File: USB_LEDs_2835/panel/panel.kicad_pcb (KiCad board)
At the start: 2 copper layers, 99.9 x 120 mm, 280 parts, among them U1 MT9284_1, U2 JL8022W-L, U3 74LVC1G04

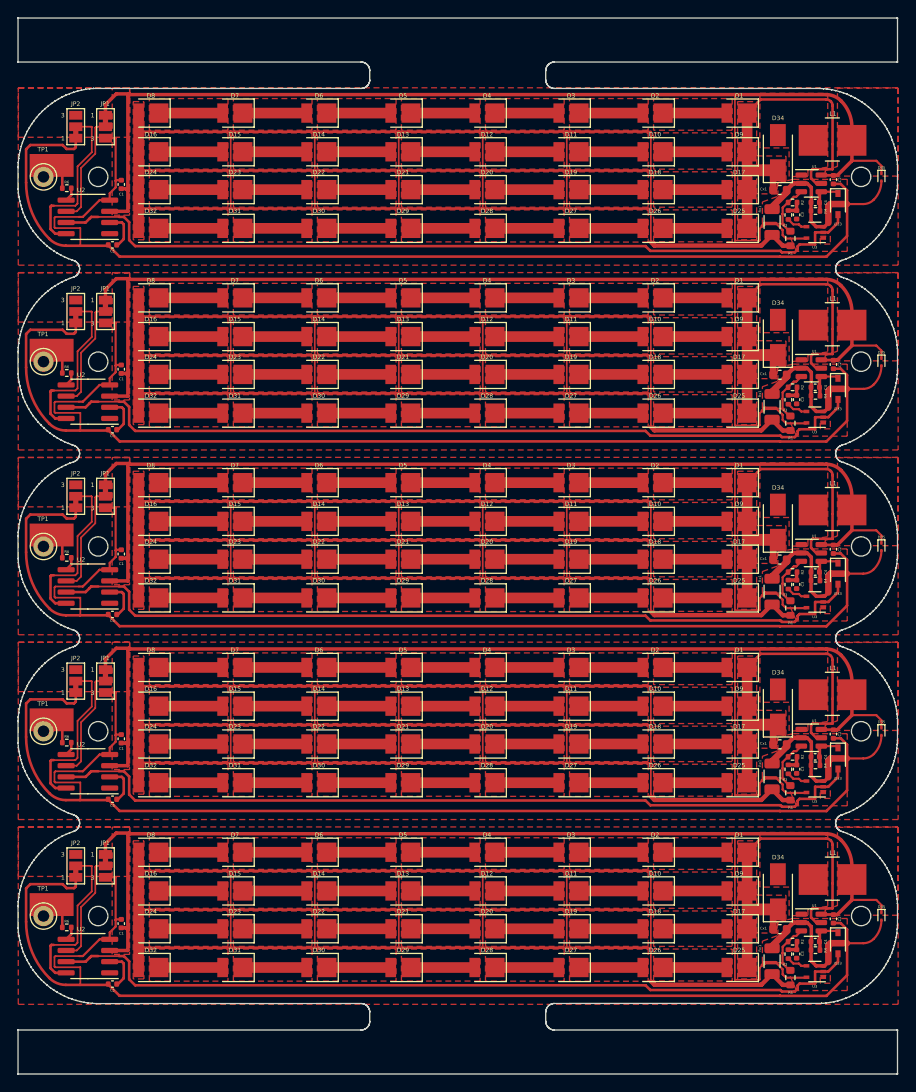
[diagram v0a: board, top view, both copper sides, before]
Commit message: Add files via upload
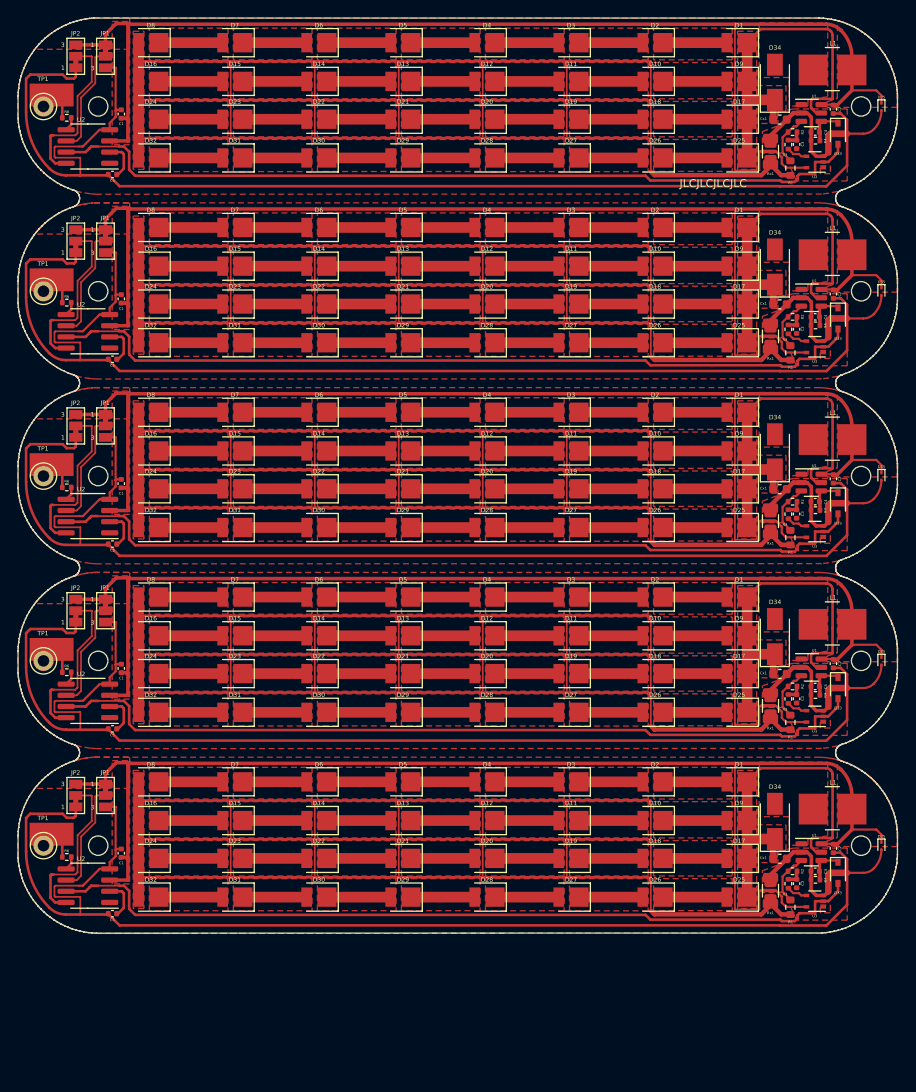
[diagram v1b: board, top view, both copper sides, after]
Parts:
- removed the C1 at (110.3, 59.9)
- removed the C1 at (110.3, 80.9)
- removed the C1 at (110.3, 38.9)
- removed the C1 at (110.3, 122.9)
- removed the C1 at (110.3, 101.9)
- removed the C2 at (191.2, 122.4)
- removed the C2 at (191.2, 38.4)
- removed the C2 at (191.2, 59.4)
- removed the C2 at (191.2, 101.4)
- removed the C2 at (191.2, 80.4)
- removed the C3 at (187.0, 63.4)
- removed the C3 at (187.0, 42.4)
- removed the C3 at (187.0, 105.4)
- removed the C3 at (187.0, 84.4)
- removed the C3 at (187.0, 126.4)
- removed the C4 at (189.1, 41.0)
- removed the C4 at (189.1, 62.0)
- removed the C4 at (189.1, 83.0)
- removed the C4 at (189.1, 104.0)
- removed the C4 at (189.1, 125.0)
- removed the C5 at (109.3, 129.8)
- removed the C5 at (109.3, 87.8)
- removed the C5 at (109.3, 108.8)
- removed the C5 at (109.3, 45.8)
- removed the C5 at (109.3, 66.8)
- removed the Cx1 at (185.1, 81.5)
- removed the Cx1 at (185.1, 123.5)
- removed the Cx1 at (185.1, 60.5)
- removed the Cx1 at (185.1, 39.5)
- removed the Cx1 at (185.1, 102.5)
- removed the D1 at (180.5, 114.8)
- removed the D1 at (180.5, 30.8)
- removed the D1 at (180.5, 72.8)
- removed the D1 at (180.5, 51.8)
- removed the D1 at (180.5, 93.8)
- removed the D10 at (170.9, 35.2)
- removed the D10 at (170.9, 77.2)
- removed the D10 at (170.9, 98.2)
- removed the D10 at (170.9, 119.2)
- removed the D10 at (170.9, 56.2)
- removed the D11 at (161.4, 35.2)
- removed the D11 at (161.4, 119.2)
- removed the D11 at (161.4, 56.2)
- removed the D11 at (161.4, 98.2)
- removed the D11 at (161.4, 77.2)
- removed the D12 at (151.8, 119.2)
- removed the D12 at (151.8, 77.2)
- removed the D12 at (151.8, 56.2)
- removed the D12 at (151.8, 98.2)
- removed the D12 at (151.8, 35.2)
- removed the D13 at (142.3, 77.2)
- removed the D13 at (142.3, 56.2)
- removed the D13 at (142.3, 98.2)
- removed the D13 at (142.3, 35.2)
- removed the D13 at (142.3, 119.2)
- removed the D14 at (132.7, 35.2)
- removed the D14 at (132.7, 98.2)
- removed the D14 at (132.7, 56.2)
- removed the D14 at (132.7, 119.2)
- removed the D14 at (132.7, 77.2)
- removed the D15 at (123.2, 119.2)
- removed the D15 at (123.2, 98.2)
- removed the D15 at (123.2, 35.2)
- removed the D15 at (123.2, 77.2)
- removed the D15 at (123.2, 56.2)
- removed the D16 at (113.6, 98.2)
- removed the D16 at (113.6, 35.2)
- removed the D16 at (113.6, 77.2)
- removed the D16 at (113.6, 56.2)
- removed the D16 at (113.6, 119.2)
- removed the D17 at (180.5, 39.5)
- removed the D17 at (180.5, 102.5)
- removed the D17 at (180.5, 123.5)
- removed the D17 at (180.5, 81.5)
- removed the D17 at (180.5, 60.5)
- removed the D18 at (170.9, 81.5)
- removed the D18 at (170.9, 123.5)
- removed the D18 at (170.9, 60.5)
- removed the D18 at (170.9, 102.5)
- removed the D18 at (170.9, 39.5)
- removed the D19 at (161.4, 123.5)
- removed the D19 at (161.4, 102.5)
- removed the D19 at (161.4, 39.5)
- removed the D19 at (161.4, 81.5)
- removed the D19 at (161.4, 60.5)
- removed the D2 at (170.9, 114.8)
- removed the D2 at (170.9, 93.8)
- removed the D2 at (170.9, 72.8)
- removed the D2 at (170.9, 51.8)
- removed the D2 at (170.9, 30.8)
- removed the D20 at (151.8, 81.5)
- removed the D20 at (151.8, 60.5)
- removed the D20 at (151.8, 102.5)
- removed the D20 at (151.8, 39.5)
- removed the D20 at (151.8, 123.5)
- removed the D21 at (142.3, 123.5)
- removed the D21 at (142.3, 39.5)
- removed the D21 at (142.3, 81.5)
- removed the D21 at (142.3, 60.5)
- removed the D21 at (142.3, 102.5)
- removed the D22 at (132.7, 39.5)
- removed the D22 at (132.7, 60.5)
- removed the D22 at (132.7, 81.5)
- removed the D22 at (132.7, 123.5)
- removed the D22 at (132.7, 102.5)
- removed the D23 at (123.2, 39.5)
- removed the D23 at (123.2, 102.5)
- removed the D23 at (123.2, 123.5)
- removed the D23 at (123.2, 81.5)
- removed the D23 at (123.2, 60.5)
- removed the D24 at (113.6, 123.5)
- removed the D24 at (113.6, 102.5)
- removed the D24 at (113.6, 60.5)
- removed the D24 at (113.6, 81.5)
- removed the D24 at (113.6, 39.5)
- removed the D25 at (180.5, 85.9)
- removed the D25 at (180.5, 43.9)
- removed the D25 at (180.5, 106.9)
- removed the D25 at (180.5, 64.9)
- removed the D25 at (180.5, 127.9)
- removed the D26 at (170.9, 106.9)
- removed the D26 at (170.9, 127.9)
- removed the D26 at (170.9, 43.9)
- removed the D26 at (170.9, 64.9)
- removed the D26 at (170.9, 85.9)
- removed the D27 at (161.4, 64.9)
- removed the D27 at (161.4, 43.9)
- removed the D27 at (161.4, 106.9)
- removed the D27 at (161.4, 127.9)
- removed the D27 at (161.4, 85.9)
- removed the D28 at (151.8, 85.9)
- removed the D28 at (151.8, 43.9)
- removed the D28 at (151.8, 106.9)
- removed the D28 at (151.8, 64.9)
- removed the D28 at (151.8, 127.9)
- removed the D29 at (142.3, 85.9)
- removed the D29 at (142.3, 64.9)
- removed the D29 at (142.3, 43.9)
- removed the D29 at (142.3, 127.9)
- removed the D29 at (142.3, 106.9)
- removed the D3 at (161.4, 51.8)
- removed the D3 at (161.4, 30.8)
- removed the D3 at (161.4, 72.8)
- removed the D3 at (161.4, 93.8)
- removed the D3 at (161.4, 114.8)
- removed the D30 at (132.7, 85.9)
- removed the D30 at (132.7, 43.9)
- removed the D30 at (132.7, 64.9)
- removed the D30 at (132.7, 106.9)
- removed the D30 at (132.7, 127.9)
- removed the D31 at (123.2, 85.9)
- removed the D31 at (123.2, 43.9)
- removed the D31 at (123.2, 106.9)
- removed the D31 at (123.2, 64.9)
- removed the D31 at (123.2, 127.9)
- removed the D32 at (113.6, 106.9)
- removed the D32 at (113.6, 127.9)
- removed the D32 at (113.6, 64.9)
- removed the D32 at (113.6, 43.9)
- removed the D32 at (113.6, 85.9)
- removed the D33 at (191.7, 83.0)
- removed the D33 at (191.7, 125.0)
- removed the D33 at (191.7, 104.0)
- removed the D33 at (191.7, 62.0)
- removed the D33 at (191.7, 41.0)
- removed the D34 at (184.9, 98.3)
- removed the D34 at (184.9, 77.3)
- removed the D34 at (184.9, 35.3)
- removed the D34 at (184.9, 56.3)
- removed the D34 at (184.9, 119.3)
- removed the D35 at (196.6, 101.1)
- removed the D35 at (196.6, 38.1)
- removed the D35 at (196.6, 122.1)
- removed the D35 at (196.6, 59.1)
- removed the D35 at (196.6, 80.1)
- removed the D4 at (151.8, 30.8)
- removed the D4 at (151.8, 72.8)
- removed the D4 at (151.8, 51.8)
- removed the D4 at (151.8, 114.8)
- removed the D4 at (151.8, 93.8)
- removed the D5 at (142.3, 93.8)
- removed the D5 at (142.3, 51.8)
- removed the D5 at (142.3, 72.8)
- removed the D5 at (142.3, 114.8)
- removed the D5 at (142.3, 30.8)
- removed the D6 at (132.7, 30.8)
- removed the D6 at (132.7, 72.8)
- removed the D6 at (132.7, 51.8)
- removed the D6 at (132.7, 93.8)
- removed the D6 at (132.7, 114.8)
- removed the D7 at (123.2, 51.8)
- removed the D7 at (123.2, 93.8)
- removed the D7 at (123.2, 114.8)
- removed the D7 at (123.2, 72.8)
- removed the D7 at (123.2, 30.8)
- removed the D8 at (113.6, 72.8)
- removed the D8 at (113.6, 93.8)
- removed the D8 at (113.6, 30.8)
- removed the D8 at (113.6, 51.8)
- removed the D8 at (113.6, 114.8)
- removed the D9 at (180.5, 119.2)
- removed the D9 at (180.5, 98.2)
- removed the D9 at (180.5, 77.2)
- removed the D9 at (180.5, 56.2)
- removed the D9 at (180.5, 35.2)
- removed the H1 at (194.3, 122.0)
- removed the H1 at (194.3, 101.0)
- removed the H1 at (194.3, 80.0)
- removed the H1 at (194.3, 59.0)
- removed the H1 at (194.3, 38.0)
- removed the H2 at (107.7, 59.0)
- removed the H2 at (107.7, 101.0)
- removed the H2 at (107.7, 122.0)
- removed the H2 at (107.7, 38.0)
- removed the H2 at (107.7, 80.0)
- removed the JP1 at (108.5, 95.3)
- removed the JP1 at (108.5, 53.3)
- removed the JP1 at (108.5, 74.3)
- removed the JP1 at (108.5, 32.3)
- removed the JP1 at (108.5, 116.3)
- removed the JP2 at (105.1, 116.3)
- removed the JP2 at (105.1, 95.3)
- removed the JP2 at (105.1, 32.3)
- removed the JP2 at (105.1, 53.3)
- removed the JP2 at (105.1, 74.3)
- removed the L1 at (191.1, 33.9)
- removed the L1 at (191.1, 96.9)
- removed the L1 at (191.1, 54.9)
- removed the L1 at (191.1, 75.9)
- removed the L1 at (191.1, 117.9)
- removed the R1 at (186.3, 108.0)
- removed the R1 at (186.3, 129.0)
- removed the R1 at (186.3, 87.0)
- removed the R1 at (186.3, 66.0)
- removed the R1 at (186.3, 45.0)
- removed the R2 at (186.5, 104.0)
- removed the R2 at (186.5, 62.0)
- removed the R2 at (186.5, 83.0)
- removed the R2 at (186.5, 125.0)
- removed the R2 at (186.5, 41.0)
- removed the R3 at (186.1, 42.4)
- removed the R3 at (186.1, 84.4)
- removed the R3 at (186.1, 126.4)
- removed the R3 at (186.1, 63.4)
- removed the R3 at (186.1, 105.4)
- removed the R4 at (189.1, 41.9)
- removed the R4 at (189.1, 62.9)
- removed the R4 at (189.1, 125.9)
- removed the R4 at (189.1, 104.9)
- removed the R4 at (189.1, 83.9)
- removed the R6 at (104.1, 102.3)
- removed the R6 at (104.1, 39.3)
- removed the R6 at (104.1, 123.3)
- removed the R6 at (104.1, 60.3)
- removed the R6 at (104.1, 81.3)
- removed the Rx1 at (184.2, 106.2)
- removed the Rx1 at (184.2, 43.2)
- removed the Rx1 at (184.2, 85.2)
- removed the Rx1 at (184.2, 127.2)
- removed the Rx1 at (184.2, 64.2)
- removed the TP1 at (101.4, 80.0)
- removed the TP1 at (101.4, 38.0)
- removed the TP1 at (101.4, 59.0)
- removed the TP1 at (101.4, 122.0)
- removed the TP1 at (101.4, 101.0)
- removed the U1 at (188.7, 80.8)
- removed the U1 at (188.7, 38.8)
- removed the U1 at (188.7, 122.8)
- removed the U1 at (188.7, 59.8)
- removed the U1 at (188.7, 101.8)
- removed the U2 at (106.5, 126.6)
- removed the U2 at (106.5, 84.6)
- removed the U2 at (106.5, 63.6)
- removed the U2 at (106.5, 105.6)
- removed the U2 at (106.5, 42.6)
- removed the U3 at (189.1, 86.4)
- removed the U3 at (189.1, 128.4)
- removed the U3 at (189.1, 44.4)
- removed the U3 at (189.1, 65.4)
- removed the U3 at (189.1, 107.4)
- added C1: 1u, Capacitor_SMD:C_0402_1005Metric, F.Cu at (110.3, 93.9)
- added C1: 1u, Capacitor_SMD:C_0402_1005Metric, F.Cu at (110.3, 51.9)
- added C1: 1u, Capacitor_SMD:C_0402_1005Metric, F.Cu at (110.3, 30.9)
- added C1: 1u, Capacitor_SMD:C_0402_1005Metric, F.Cu at (110.3, 114.9)
- added C1: 1u, Capacitor_SMD:C_0402_1005Metric, F.Cu at (110.3, 72.9)
- added C2: 22u, Capacitor_SMD:C_0402_1005Metric, F.Cu at (191.2, 30.4)
- added C2: 22u, Capacitor_SMD:C_0402_1005Metric, F.Cu at (191.2, 93.4)
- added C2: 22u, Capacitor_SMD:C_0402_1005Metric, F.Cu at (191.2, 114.4)
- added C2: 22u, Capacitor_SMD:C_0402_1005Metric, F.Cu at (191.2, 51.4)
- added C2: 22u, Capacitor_SMD:C_0402_1005Metric, F.Cu at (191.2, 72.4)
- added C3: 1u, Capacitor_SMD:C_0402_1005Metric, F.Cu at (187.0, 55.4)
- added C3: 1u, Capacitor_SMD:C_0402_1005Metric, F.Cu at (187.0, 34.4)
- added C3: 1u, Capacitor_SMD:C_0402_1005Metric, F.Cu at (187.0, 118.4)
- added C3: 1u, Capacitor_SMD:C_0402_1005Metric, F.Cu at (187.0, 76.4)
- added C3: 1u, Capacitor_SMD:C_0402_1005Metric, F.Cu at (187.0, 97.4)
- added C4: 1n, Capacitor_SMD:C_0402_1005Metric, F.Cu at (189.1, 96.0)
- added C4: 1n, Capacitor_SMD:C_0402_1005Metric, F.Cu at (189.1, 117.0)
- added C4: 1n, Capacitor_SMD:C_0402_1005Metric, F.Cu at (189.1, 75.0)
- added C4: 1n, Capacitor_SMD:C_0402_1005Metric, F.Cu at (189.1, 33.0)
- added C4: 1n, Capacitor_SMD:C_0402_1005Metric, F.Cu at (189.1, 54.0)
- added C5: 10n, Capacitor_SMD:C_0402_1005Metric, F.Cu at (109.3, 121.8)
- added C5: 10n, Capacitor_SMD:C_0402_1005Metric, F.Cu at (109.3, 100.8)
- added C5: 10n, Capacitor_SMD:C_0402_1005Metric, F.Cu at (109.3, 37.8)
- added C5: 10n, Capacitor_SMD:C_0402_1005Metric, F.Cu at (109.3, 58.8)
- added C5: 10n, Capacitor_SMD:C_0402_1005Metric, F.Cu at (109.3, 79.8)
- added Cx1: 22u, Capacitor_SMD:C_0603_1608Metric, F.Cu at (185.1, 94.5)
- added Cx1: 22u, Capacitor_SMD:C_0603_1608Metric, F.Cu at (185.1, 31.5)
- added Cx1: 22u, Capacitor_SMD:C_0603_1608Metric, F.Cu at (185.1, 73.5)
- added Cx1: 22u, Capacitor_SMD:C_0603_1608Metric, F.Cu at (185.1, 115.5)
- added Cx1: 22u, Capacitor_SMD:C_0603_1608Metric, F.Cu at (185.1, 52.5)
- added D1: 660nm, LED_SMD:LED_2835_custom_margin, F.Cu at (180.5, 106.8)
- added D1: 660nm, LED_SMD:LED_2835_custom_margin, F.Cu at (180.5, 22.8)
- added D1: 660nm, LED_SMD:LED_2835_custom_margin, F.Cu at (180.5, 85.8)
- added D1: 660nm, LED_SMD:LED_2835_custom_margin, F.Cu at (180.5, 43.8)
- added D1: 660nm, LED_SMD:LED_2835_custom_margin, F.Cu at (180.5, 64.8)
- added D10: 660nm, LED_SMD:LED_2835_custom_margin, F.Cu at (170.9, 27.2)
- added D10: 660nm, LED_SMD:LED_2835_custom_margin, F.Cu at (170.9, 48.2)
- added D10: 660nm, LED_SMD:LED_2835_custom_margin, F.Cu at (170.9, 69.2)
- added D10: 660nm, LED_SMD:LED_2835_custom_margin, F.Cu at (170.9, 90.2)
- added D10: 660nm, LED_SMD:LED_2835_custom_margin, F.Cu at (170.9, 111.2)
- added D11: 660nm, LED_SMD:LED_2835_custom_margin, F.Cu at (161.4, 48.2)
- added D11: 660nm, LED_SMD:LED_2835_custom_margin, F.Cu at (161.4, 27.2)
- added D11: 660nm, LED_SMD:LED_2835_custom_margin, F.Cu at (161.4, 111.2)
- added D11: 660nm, LED_SMD:LED_2835_custom_margin, F.Cu at (161.4, 90.2)
- added D11: 660nm, LED_SMD:LED_2835_custom_margin, F.Cu at (161.4, 69.2)
- added D12: 660nm, LED_SMD:LED_2835_custom_margin, F.Cu at (151.8, 27.2)
- added D12: 660nm, LED_SMD:LED_2835_custom_margin, F.Cu at (151.8, 90.2)
- added D12: 660nm, LED_SMD:LED_2835_custom_margin, F.Cu at (151.8, 111.2)
- added D12: 660nm, LED_SMD:LED_2835_custom_margin, F.Cu at (151.8, 69.2)
- added D12: 660nm, LED_SMD:LED_2835_custom_margin, F.Cu at (151.8, 48.2)
- added D13: 660nm, LED_SMD:LED_2835_custom_margin, F.Cu at (142.3, 48.2)
- added D13: 660nm, LED_SMD:LED_2835_custom_margin, F.Cu at (142.3, 69.2)
- added D13: 660nm, LED_SMD:LED_2835_custom_margin, F.Cu at (142.3, 90.2)
- added D13: 660nm, LED_SMD:LED_2835_custom_margin, F.Cu at (142.3, 27.2)
- added D13: 660nm, LED_SMD:LED_2835_custom_margin, F.Cu at (142.3, 111.2)
- added D14: 660nm, LED_SMD:LED_2835_custom_margin, F.Cu at (132.7, 111.2)
- added D14: 660nm, LED_SMD:LED_2835_custom_margin, F.Cu at (132.7, 48.2)
- added D14: 660nm, LED_SMD:LED_2835_custom_margin, F.Cu at (132.7, 69.2)
- added D14: 660nm, LED_SMD:LED_2835_custom_margin, F.Cu at (132.7, 90.2)
- added D14: 660nm, LED_SMD:LED_2835_custom_margin, F.Cu at (132.7, 27.2)
- added D15: 660nm, LED_SMD:LED_2835_custom_margin, F.Cu at (123.2, 69.2)
- added D15: 660nm, LED_SMD:LED_2835_custom_margin, F.Cu at (123.2, 48.2)
- added D15: 660nm, LED_SMD:LED_2835_custom_margin, F.Cu at (123.2, 27.2)
- added D15: 660nm, LED_SMD:LED_2835_custom_margin, F.Cu at (123.2, 90.2)
- added D15: 660nm, LED_SMD:LED_2835_custom_margin, F.Cu at (123.2, 111.2)
- added D16: 660nm, LED_SMD:LED_2835_custom_margin, F.Cu at (113.6, 111.2)
- added D16: 660nm, LED_SMD:LED_2835_custom_margin, F.Cu at (113.6, 69.2)
- added D16: 660nm, LED_SMD:LED_2835_custom_margin, F.Cu at (113.6, 27.2)
- added D16: 660nm, LED_SMD:LED_2835_custom_margin, F.Cu at (113.6, 90.2)
- added D16: 660nm, LED_SMD:LED_2835_custom_margin, F.Cu at (113.6, 48.2)
- added D17: 660nm, LED_SMD:LED_2835_custom_margin, F.Cu at (180.5, 115.5)
- added D17: 660nm, LED_SMD:LED_2835_custom_margin, F.Cu at (180.5, 73.5)
- added D17: 660nm, LED_SMD:LED_2835_custom_margin, F.Cu at (180.5, 31.5)
- added D17: 660nm, LED_SMD:LED_2835_custom_margin, F.Cu at (180.5, 94.5)
- added D17: 660nm, LED_SMD:LED_2835_custom_margin, F.Cu at (180.5, 52.5)
- added D18: 660nm, LED_SMD:LED_2835_custom_margin, F.Cu at (170.9, 31.5)
- added D18: 660nm, LED_SMD:LED_2835_custom_margin, F.Cu at (170.9, 94.5)
- added D18: 660nm, LED_SMD:LED_2835_custom_margin, F.Cu at (170.9, 52.5)
- added D18: 660nm, LED_SMD:LED_2835_custom_margin, F.Cu at (170.9, 115.5)
- added D18: 660nm, LED_SMD:LED_2835_custom_margin, F.Cu at (170.9, 73.5)
- added D19: 660nm, LED_SMD:LED_2835_custom_margin, F.Cu at (161.4, 115.5)
- added D19: 660nm, LED_SMD:LED_2835_custom_margin, F.Cu at (161.4, 52.5)
- added D19: 660nm, LED_SMD:LED_2835_custom_margin, F.Cu at (161.4, 31.5)
- added D19: 660nm, LED_SMD:LED_2835_custom_margin, F.Cu at (161.4, 94.5)
- added D19: 660nm, LED_SMD:LED_2835_custom_margin, F.Cu at (161.4, 73.5)
- added D2: 660nm, LED_SMD:LED_2835_custom_margin, F.Cu at (170.9, 43.8)
- added D2: 660nm, LED_SMD:LED_2835_custom_margin, F.Cu at (170.9, 85.8)
- added D2: 660nm, LED_SMD:LED_2835_custom_margin, F.Cu at (170.9, 64.8)
- added D2: 660nm, LED_SMD:LED_2835_custom_margin, F.Cu at (170.9, 106.8)
- added D2: 660nm, LED_SMD:LED_2835_custom_margin, F.Cu at (170.9, 22.8)
- added D20: 660nm, LED_SMD:LED_2835_custom_margin, F.Cu at (151.8, 52.5)
- added D20: 660nm, LED_SMD:LED_2835_custom_margin, F.Cu at (151.8, 73.5)
- added D20: 660nm, LED_SMD:LED_2835_custom_margin, F.Cu at (151.8, 31.5)
- added D20: 660nm, LED_SMD:LED_2835_custom_margin, F.Cu at (151.8, 115.5)
- added D20: 660nm, LED_SMD:LED_2835_custom_margin, F.Cu at (151.8, 94.5)
- added D21: 660nm, LED_SMD:LED_2835_custom_margin, F.Cu at (142.3, 73.5)
- added D21: 660nm, LED_SMD:LED_2835_custom_margin, F.Cu at (142.3, 115.5)
- added D21: 660nm, LED_SMD:LED_2835_custom_margin, F.Cu at (142.3, 52.5)
- added D21: 660nm, LED_SMD:LED_2835_custom_margin, F.Cu at (142.3, 94.5)
- added D21: 660nm, LED_SMD:LED_2835_custom_margin, F.Cu at (142.3, 31.5)
- added D22: 660nm, LED_SMD:LED_2835_custom_margin, F.Cu at (132.7, 94.5)
- added D22: 660nm, LED_SMD:LED_2835_custom_margin, F.Cu at (132.7, 115.5)
- added D22: 660nm, LED_SMD:LED_2835_custom_margin, F.Cu at (132.7, 31.5)
- added D22: 660nm, LED_SMD:LED_2835_custom_margin, F.Cu at (132.7, 52.5)
- added D22: 660nm, LED_SMD:LED_2835_custom_margin, F.Cu at (132.7, 73.5)
- added D23: 660nm, LED_SMD:LED_2835_custom_margin, F.Cu at (123.2, 73.5)
- added D23: 660nm, LED_SMD:LED_2835_custom_margin, F.Cu at (123.2, 94.5)
- added D23: 660nm, LED_SMD:LED_2835_custom_margin, F.Cu at (123.2, 115.5)
- added D23: 660nm, LED_SMD:LED_2835_custom_margin, F.Cu at (123.2, 31.5)
- added D23: 660nm, LED_SMD:LED_2835_custom_margin, F.Cu at (123.2, 52.5)
- added D24: 660nm, LED_SMD:LED_2835_custom_margin, F.Cu at (113.6, 73.5)
- added D24: 660nm, LED_SMD:LED_2835_custom_margin, F.Cu at (113.6, 115.5)
- added D24: 660nm, LED_SMD:LED_2835_custom_margin, F.Cu at (113.6, 31.5)
- added D24: 660nm, LED_SMD:LED_2835_custom_margin, F.Cu at (113.6, 52.5)
- added D24: 660nm, LED_SMD:LED_2835_custom_margin, F.Cu at (113.6, 94.5)
- added D25: 660nm, LED_SMD:LED_2835_custom_margin, F.Cu at (180.5, 98.9)
- added D25: 660nm, LED_SMD:LED_2835_custom_margin, F.Cu at (180.5, 35.9)
- added D25: 660nm, LED_SMD:LED_2835_custom_margin, F.Cu at (180.5, 56.9)
- added D25: 660nm, LED_SMD:LED_2835_custom_margin, F.Cu at (180.5, 119.9)
- added D25: 660nm, LED_SMD:LED_2835_custom_margin, F.Cu at (180.5, 77.9)
- added D26: 660nm, LED_SMD:LED_2835_custom_margin, F.Cu at (170.9, 56.9)
- added D26: 660nm, LED_SMD:LED_2835_custom_margin, F.Cu at (170.9, 119.9)
- added D26: 660nm, LED_SMD:LED_2835_custom_margin, F.Cu at (170.9, 35.9)
- added D26: 660nm, LED_SMD:LED_2835_custom_margin, F.Cu at (170.9, 98.9)
- added D26: 660nm, LED_SMD:LED_2835_custom_margin, F.Cu at (170.9, 77.9)
- added D27: 660nm, LED_SMD:LED_2835_custom_margin, F.Cu at (161.4, 98.9)
- added D27: 660nm, LED_SMD:LED_2835_custom_margin, F.Cu at (161.4, 77.9)
- added D27: 660nm, LED_SMD:LED_2835_custom_margin, F.Cu at (161.4, 35.9)
- added D27: 660nm, LED_SMD:LED_2835_custom_margin, F.Cu at (161.4, 119.9)
- added D27: 660nm, LED_SMD:LED_2835_custom_margin, F.Cu at (161.4, 56.9)
- added D28: 660nm, LED_SMD:LED_2835_custom_margin, F.Cu at (151.8, 35.9)
- added D28: 660nm, LED_SMD:LED_2835_custom_margin, F.Cu at (151.8, 77.9)
- added D28: 660nm, LED_SMD:LED_2835_custom_margin, F.Cu at (151.8, 56.9)
- added D28: 660nm, LED_SMD:LED_2835_custom_margin, F.Cu at (151.8, 119.9)
- added D28: 660nm, LED_SMD:LED_2835_custom_margin, F.Cu at (151.8, 98.9)
- added D29: 660nm, LED_SMD:LED_2835_custom_margin, F.Cu at (142.3, 35.9)
- added D29: 660nm, LED_SMD:LED_2835_custom_margin, F.Cu at (142.3, 77.9)
- added D29: 660nm, LED_SMD:LED_2835_custom_margin, F.Cu at (142.3, 98.9)
- added D29: 660nm, LED_SMD:LED_2835_custom_margin, F.Cu at (142.3, 119.9)
- added D29: 660nm, LED_SMD:LED_2835_custom_margin, F.Cu at (142.3, 56.9)
- added D3: 660nm, LED_SMD:LED_2835_custom_margin, F.Cu at (161.4, 64.8)
- added D3: 660nm, LED_SMD:LED_2835_custom_margin, F.Cu at (161.4, 106.8)
- added D3: 660nm, LED_SMD:LED_2835_custom_margin, F.Cu at (161.4, 43.8)
- added D3: 660nm, LED_SMD:LED_2835_custom_margin, F.Cu at (161.4, 85.8)
- added D3: 660nm, LED_SMD:LED_2835_custom_margin, F.Cu at (161.4, 22.8)
- added D30: 660nm, LED_SMD:LED_2835_custom_margin, F.Cu at (132.7, 98.9)
- added D30: 660nm, LED_SMD:LED_2835_custom_margin, F.Cu at (132.7, 56.9)
- added D30: 660nm, LED_SMD:LED_2835_custom_margin, F.Cu at (132.7, 77.9)
- added D30: 660nm, LED_SMD:LED_2835_custom_margin, F.Cu at (132.7, 35.9)
- added D30: 660nm, LED_SMD:LED_2835_custom_margin, F.Cu at (132.7, 119.9)
- added D31: 660nm, LED_SMD:LED_2835_custom_margin, F.Cu at (123.2, 56.9)
- added D31: 660nm, LED_SMD:LED_2835_custom_margin, F.Cu at (123.2, 35.9)
- added D31: 660nm, LED_SMD:LED_2835_custom_margin, F.Cu at (123.2, 77.9)
- added D31: 660nm, LED_SMD:LED_2835_custom_margin, F.Cu at (123.2, 98.9)
- added D31: 660nm, LED_SMD:LED_2835_custom_margin, F.Cu at (123.2, 119.9)
- added D32: 660nm, LED_SMD:LED_2835_custom_margin, F.Cu at (113.6, 77.9)
- added D32: 660nm, LED_SMD:LED_2835_custom_margin, F.Cu at (113.6, 35.9)
- added D32: 660nm, LED_SMD:LED_2835_custom_margin, F.Cu at (113.6, 56.9)
- added D32: 660nm, LED_SMD:LED_2835_custom_margin, F.Cu at (113.6, 98.9)
- added D32: 660nm, LED_SMD:LED_2835_custom_margin, F.Cu at (113.6, 119.9)
- added D33: 1N4148WS, Diode_SMD:D_SOD-323_custom, F.Cu at (191.7, 54.0)
- added D33: 1N4148WS, Diode_SMD:D_SOD-323_custom, F.Cu at (191.7, 75.0)
- added D33: 1N4148WS, Diode_SMD:D_SOD-323_custom, F.Cu at (191.7, 117.0)
- added D33: 1N4148WS, Diode_SMD:D_SOD-323_custom, F.Cu at (191.7, 33.0)
- added D33: 1N4148WS, Diode_SMD:D_SOD-323_custom, F.Cu at (191.7, 96.0)
- added D34: SS14, Diode_SMD:D_SMA, F.Cu at (184.5, 90.3)
- added D34: SS14, Diode_SMD:D_SMA, F.Cu at (184.5, 69.3)
- added D34: SS14, Diode_SMD:D_SMA, F.Cu at (184.5, 111.3)
- added D34: SS14, Diode_SMD:D_SMA, F.Cu at (184.5, 27.3)
- added D34: SS14, Diode_SMD:D_SMA, F.Cu at (184.5, 48.3)
- added D35: D_TVS_unidirection, Diode_SMD:D_SOD-923, F.Cu at (196.6, 51.1)
- added D35: D_TVS_unidirection, Diode_SMD:D_SOD-923, F.Cu at (196.6, 72.1)
- added D35: D_TVS_unidirection, Diode_SMD:D_SOD-923, F.Cu at (196.6, 93.1)
- added D35: D_TVS_unidirection, Diode_SMD:D_SOD-923, F.Cu at (196.6, 114.1)
- added D35: D_TVS_unidirection, Diode_SMD:D_SOD-923, F.Cu at (196.6, 30.1)
- added D4: 660nm, LED_SMD:LED_2835_custom_margin, F.Cu at (151.8, 85.8)
- added D4: 660nm, LED_SMD:LED_2835_custom_margin, F.Cu at (151.8, 64.8)
- added D4: 660nm, LED_SMD:LED_2835_custom_margin, F.Cu at (151.8, 106.8)
- added D4: 660nm, LED_SMD:LED_2835_custom_margin, F.Cu at (151.8, 22.8)
- added D4: 660nm, LED_SMD:LED_2835_custom_margin, F.Cu at (151.8, 43.8)
- added D5: 660nm, LED_SMD:LED_2835_custom_margin, F.Cu at (142.3, 43.8)
- added D5: 660nm, LED_SMD:LED_2835_custom_margin, F.Cu at (142.3, 85.8)
- added D5: 660nm, LED_SMD:LED_2835_custom_margin, F.Cu at (142.3, 64.8)
- added D5: 660nm, LED_SMD:LED_2835_custom_margin, F.Cu at (142.3, 22.8)
- added D5: 660nm, LED_SMD:LED_2835_custom_margin, F.Cu at (142.3, 106.8)
- added D6: 660nm, LED_SMD:LED_2835_custom_margin, F.Cu at (132.7, 64.8)
- added D6: 660nm, LED_SMD:LED_2835_custom_margin, F.Cu at (132.7, 22.8)
- added D6: 660nm, LED_SMD:LED_2835_custom_margin, F.Cu at (132.7, 106.8)
- added D6: 660nm, LED_SMD:LED_2835_custom_margin, F.Cu at (132.7, 43.8)
- added D6: 660nm, LED_SMD:LED_2835_custom_margin, F.Cu at (132.7, 85.8)
- added D7: 660nm, LED_SMD:LED_2835_custom_margin, F.Cu at (123.2, 85.8)
- added D7: 660nm, LED_SMD:LED_2835_custom_margin, F.Cu at (123.2, 106.8)
- added D7: 660nm, LED_SMD:LED_2835_custom_margin, F.Cu at (123.2, 43.8)
- added D7: 660nm, LED_SMD:LED_2835_custom_margin, F.Cu at (123.2, 22.8)
- added D7: 660nm, LED_SMD:LED_2835_custom_margin, F.Cu at (123.2, 64.8)
- added D8: 660nm, LED_SMD:LED_2835_custom_margin, F.Cu at (113.6, 22.8)
- added D8: 660nm, LED_SMD:LED_2835_custom_margin, F.Cu at (113.6, 85.8)
- added D8: 660nm, LED_SMD:LED_2835_custom_margin, F.Cu at (113.6, 64.8)
- added D8: 660nm, LED_SMD:LED_2835_custom_margin, F.Cu at (113.6, 43.8)
- added D8: 660nm, LED_SMD:LED_2835_custom_margin, F.Cu at (113.6, 106.8)
- added D9: 660nm, LED_SMD:LED_2835_custom_margin, F.Cu at (180.5, 69.2)
- added D9: 660nm, LED_SMD:LED_2835_custom_margin, F.Cu at (180.5, 27.2)
- added D9: 660nm, LED_SMD:LED_2835_custom_margin, F.Cu at (180.5, 48.2)
- added D9: 660nm, LED_SMD:LED_2835_custom_margin, F.Cu at (180.5, 111.2)
- added D9: 660nm, LED_SMD:LED_2835_custom_margin, F.Cu at (180.5, 90.2)
- added H1: MountingHole, MountingHole:MountingHole_2.1mm, F.Cu at (194.3, 51.0)
- added H1: MountingHole, MountingHole:MountingHole_2.1mm, F.Cu at (194.3, 114.0)
- added H1: MountingHole, MountingHole:MountingHole_2.1mm, F.Cu at (194.3, 93.0)
- added H1: MountingHole, MountingHole:MountingHole_2.1mm, F.Cu at (194.3, 72.0)
- added H1: MountingHole, MountingHole:MountingHole_2.1mm, F.Cu at (194.3, 30.0)
- added H2: MountingHole, MountingHole:MountingHole_2.1mm, F.Cu at (107.7, 114.0)
- added H2: MountingHole, MountingHole:MountingHole_2.1mm, F.Cu at (107.7, 30.0)
- added H2: MountingHole, MountingHole:MountingHole_2.1mm, F.Cu at (107.7, 93.0)
- added H2: MountingHole, MountingHole:MountingHole_2.1mm, F.Cu at (107.7, 51.0)
- added H2: MountingHole, MountingHole:MountingHole_2.1mm, F.Cu at (107.7, 72.0)
- added JP1: solderjumper_1, Jumper:SolderJumper-3_P1.3mm_Bridged12_Pad1.0x1.5mm_NumberLabels, F.Cu at (108.5, 108.3)
- added JP1: solderjumper_1, Jumper:SolderJumper-3_P1.3mm_Bridged12_Pad1.0x1.5mm_NumberLabels, F.Cu at (108.5, 24.3)
- added JP1: solderjumper_1, Jumper:SolderJumper-3_P1.3mm_Bridged12_Pad1.0x1.5mm_NumberLabels, F.Cu at (108.5, 66.3)
- added JP1: solderjumper_1, Jumper:SolderJumper-3_P1.3mm_Bridged12_Pad1.0x1.5mm_NumberLabels, F.Cu at (108.5, 45.3)
- added JP1: solderjumper_1, Jumper:SolderJumper-3_P1.3mm_Bridged12_Pad1.0x1.5mm_NumberLabels, F.Cu at (108.5, 87.3)
- added JP2: solderjumper_2, Jumper:SolderJumper-3_P1.3mm_Bridged12_Pad1.0x1.5mm_NumberLabels, F.Cu at (105.1, 45.3)
- added JP2: solderjumper_2, Jumper:SolderJumper-3_P1.3mm_Bridged12_Pad1.0x1.5mm_NumberLabels, F.Cu at (105.1, 108.3)
- added JP2: solderjumper_2, Jumper:SolderJumper-3_P1.3mm_Bridged12_Pad1.0x1.5mm_NumberLabels, F.Cu at (105.1, 87.3)
- added JP2: solderjumper_2, Jumper:SolderJumper-3_P1.3mm_Bridged12_Pad1.0x1.5mm_NumberLabels, F.Cu at (105.1, 24.3)
- added JP2: solderjumper_2, Jumper:SolderJumper-3_P1.3mm_Bridged12_Pad1.0x1.5mm_NumberLabels, F.Cu at (105.1, 66.3)
- added L1: L_Ferrite_Small, custom_footprint_library:L_WHC_0630_custom, F.Cu at (191.1, 67.9)
- added L1: L_Ferrite_Small, custom_footprint_library:L_WHC_0630_custom, F.Cu at (191.1, 109.9)
- added L1: L_Ferrite_Small, custom_footprint_library:L_WHC_0630_custom, F.Cu at (191.1, 25.9)
- added L1: L_Ferrite_Small, custom_footprint_library:L_WHC_0630_custom, F.Cu at (191.1, 88.9)
- added L1: L_Ferrite_Small, custom_footprint_library:L_WHC_0630_custom, F.Cu at (191.1, 46.9)
- added R1: 23.2k, Resistor_SMD:R_0603_1608Metric, F.Cu at (186.3, 100.0)
- added R1: 23.2k, Resistor_SMD:R_0603_1608Metric, F.Cu at (186.3, 37.0)
- added R1: 23.2k, Resistor_SMD:R_0603_1608Metric, F.Cu at (186.3, 121.0)
- added R1: 23.2k, Resistor_SMD:R_0603_1608Metric, F.Cu at (186.3, 58.0)
- added R1: 23.2k, Resistor_SMD:R_0603_1608Metric, F.Cu at (186.3, 79.0)
- added R2: 200k, Resistor_SMD:R_0402_1005Metric, F.Cu at (186.5, 96.0)
- added R2: 200k, Resistor_SMD:R_0402_1005Metric, F.Cu at (186.5, 54.0)
- added R2: 200k, Resistor_SMD:R_0402_1005Metric, F.Cu at (186.5, 33.0)
- added R2: 200k, Resistor_SMD:R_0402_1005Metric, F.Cu at (186.5, 75.0)
- added R2: 200k, Resistor_SMD:R_0402_1005Metric, F.Cu at (186.5, 117.0)
- added R3: 200k, Resistor_SMD:R_0402_1005Metric, F.Cu at (186.1, 34.4)
- added R3: 200k, Resistor_SMD:R_0402_1005Metric, F.Cu at (186.1, 118.4)
- added R3: 200k, Resistor_SMD:R_0402_1005Metric, F.Cu at (186.1, 76.4)
- added R3: 200k, Resistor_SMD:R_0402_1005Metric, F.Cu at (186.1, 55.4)
- added R3: 200k, Resistor_SMD:R_0402_1005Metric, F.Cu at (186.1, 97.4)
- added R4: 100k, Resistor_SMD:R_0402_1005Metric, F.Cu at (189.1, 33.9)
- added R4: 100k, Resistor_SMD:R_0402_1005Metric, F.Cu at (189.1, 54.9)
- added R4: 100k, Resistor_SMD:R_0402_1005Metric, F.Cu at (189.1, 75.9)
- added R4: 100k, Resistor_SMD:R_0402_1005Metric, F.Cu at (189.1, 117.9)
- added R4: 100k, Resistor_SMD:R_0402_1005Metric, F.Cu at (189.1, 96.9)
- added R6: 5k, Resistor_SMD:R_0402_1005Metric, F.Cu at (104.1, 73.3)
- added R6: 5k, Resistor_SMD:R_0402_1005Metric, F.Cu at (104.1, 31.3)
- added R6: 5k, Resistor_SMD:R_0402_1005Metric, F.Cu at (104.1, 115.3)
- added R6: 5k, Resistor_SMD:R_0402_1005Metric, F.Cu at (104.1, 52.3)
- added R6: 5k, Resistor_SMD:R_0402_1005Metric, F.Cu at (104.1, 94.3)
- added Rx1: 1.5, custom_footprint_library:R_1206_0805_3216Metric_custom, F.Cu at (184.0, 119.2)
- added Rx1: 1.5, custom_footprint_library:R_1206_0805_3216Metric_custom, F.Cu at (184.0, 56.2)
- added Rx1: 1.5, custom_footprint_library:R_1206_0805_3216Metric_custom, F.Cu at (184.0, 98.2)
- added Rx1: 1.5, custom_footprint_library:R_1206_0805_3216Metric_custom, F.Cu at (184.0, 35.2)
- added Rx1: 1.5, custom_footprint_library:R_1206_0805_3216Metric_custom, F.Cu at (184.0, 77.2)
- added TP1: TestPoint, TestPoint:TestPoint_Loop_D2.50mm_Drill1.0mm_overlap_pad_custom, F.Cu at (101.4, 30.0)
- added TP1: TestPoint, TestPoint:TestPoint_Loop_D2.50mm_Drill1.0mm_overlap_pad_custom, F.Cu at (101.4, 72.0)
- added TP1: TestPoint, TestPoint:TestPoint_Loop_D2.50mm_Drill1.0mm_overlap_pad_custom, F.Cu at (101.4, 93.0)
- added TP1: TestPoint, TestPoint:TestPoint_Loop_D2.50mm_Drill1.0mm_overlap_pad_custom, F.Cu at (101.4, 114.0)
- added TP1: TestPoint, TestPoint:TestPoint_Loop_D2.50mm_Drill1.0mm_overlap_pad_custom, F.Cu at (101.4, 51.0)
- added U1: MT9284_1, Package_TO_SOT_SMD:SOT-23-6, F.Cu at (188.7, 72.8)
- added U1: MT9284_1, Package_TO_SOT_SMD:SOT-23-6, F.Cu at (188.7, 93.8)
- added U1: MT9284_1, Package_TO_SOT_SMD:SOT-23-6, F.Cu at (188.7, 30.8)
- added U1: MT9284_1, Package_TO_SOT_SMD:SOT-23-6, F.Cu at (188.7, 51.8)
- added U1: MT9284_1, Package_TO_SOT_SMD:SOT-23-6, F.Cu at (188.7, 114.8)
- added U2: JL8022W-L, Package_SO:SOIC-8_3.9x4.9mm_P1.27mm, F.Cu at (106.5, 97.6)
- added U2: JL8022W-L, Package_SO:SOIC-8_3.9x4.9mm_P1.27mm, F.Cu at (106.5, 76.6)
- added U2: JL8022W-L, Package_SO:SOIC-8_3.9x4.9mm_P1.27mm, F.Cu at (106.5, 34.6)
- added U2: JL8022W-L, Package_SO:SOIC-8_3.9x4.9mm_P1.27mm, F.Cu at (106.5, 55.6)
- added U2: JL8022W-L, Package_SO:SOIC-8_3.9x4.9mm_P1.27mm, F.Cu at (106.5, 118.6)
- added U3: 74LVC1G04, Package_TO_SOT_SMD:SOT-353_SC-70-5, F.Cu at (189.1, 78.4)
- added U3: 74LVC1G04, Package_TO_SOT_SMD:SOT-353_SC-70-5, F.Cu at (189.1, 120.4)
- added U3: 74LVC1G04, Package_TO_SOT_SMD:SOT-353_SC-70-5, F.Cu at (189.1, 36.4)
- added U3: 74LVC1G04, Package_TO_SOT_SMD:SOT-353_SC-70-5, F.Cu at (189.1, 57.4)
- added U3: 74LVC1G04, Package_TO_SOT_SMD:SOT-353_SC-70-5, F.Cu at (189.1, 99.4)
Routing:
- net Board_0-+5V: track 145.1 -> 149.2 mm
- net Board_4-+5V: track 145.1 -> 149.2 mm
- net Board_3-+5V: track 145.1 -> 149.2 mm
- net Board_2-+5V: track 145.1 -> 149.2 mm
- net Board_1-+5V: track 145.1 -> 149.2 mm
- net Board_3-Net-(D16-Pad1): track 259.3 -> 260.0 mm
- net Board_4-Net-(D16-Pad1): track 259.3 -> 260.0 mm
- net Board_2-Net-(D16-Pad1): track 259.3 -> 260.0 mm
- net Board_1-Net-(D16-Pad1): track 259.3 -> 260.0 mm
- net Board_0-Net-(D16-Pad1): track 259.3 -> 260.0 mm
- net Board_4-GND: track 161.7 -> 162.3 mm
- net Board_1-GND: track 161.7 -> 162.3 mm
- net Board_3-GND: track 161.7 -> 162.3 mm
- net Board_2-GND: track 161.7 -> 162.3 mm
- net Board_0-GND: track 161.7 -> 162.3 mm
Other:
- board size 99.9 x 120 mm -> 99.9 x 104 mm
- board text added: "JLCJLCJLCJLC"
